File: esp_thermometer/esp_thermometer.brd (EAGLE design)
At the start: 50 x 50 mm, 11 parts, among them U2 DS18B20

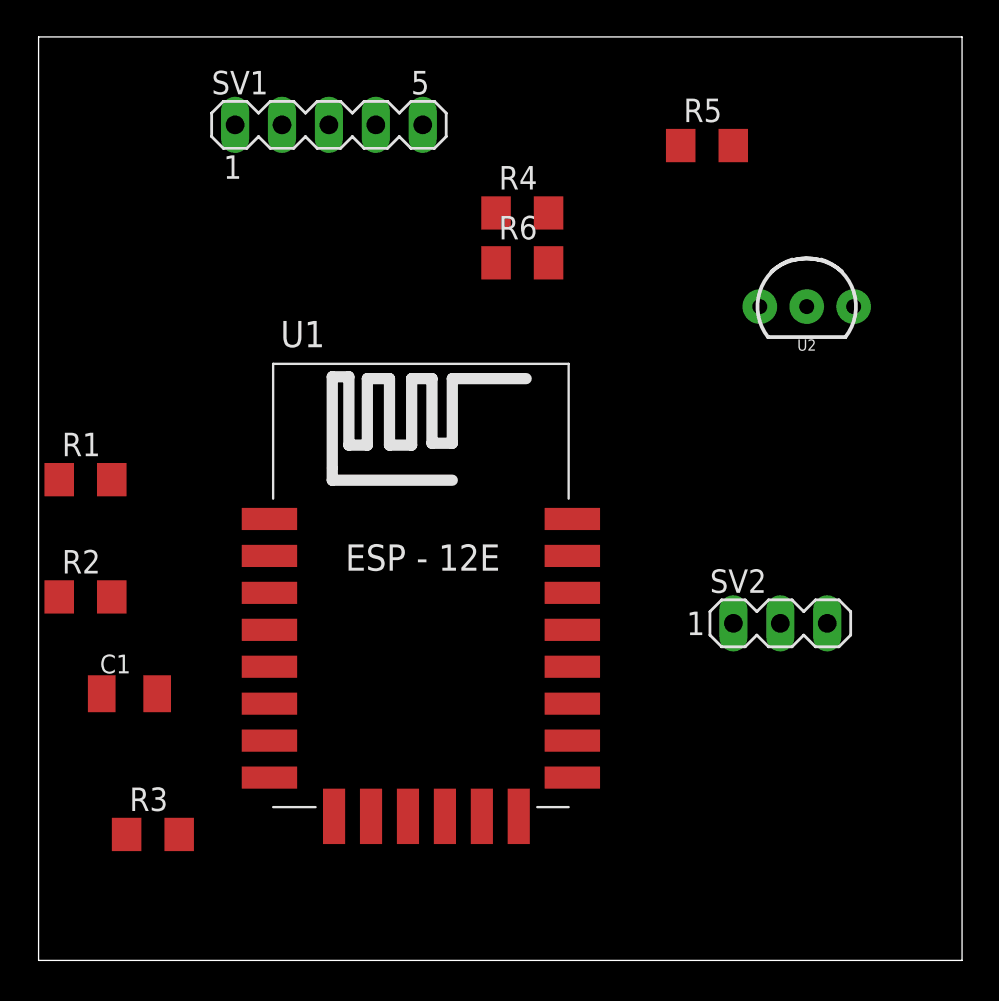
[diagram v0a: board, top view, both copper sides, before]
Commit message: Fertiger Schaltplan und Layout esp-thermometer
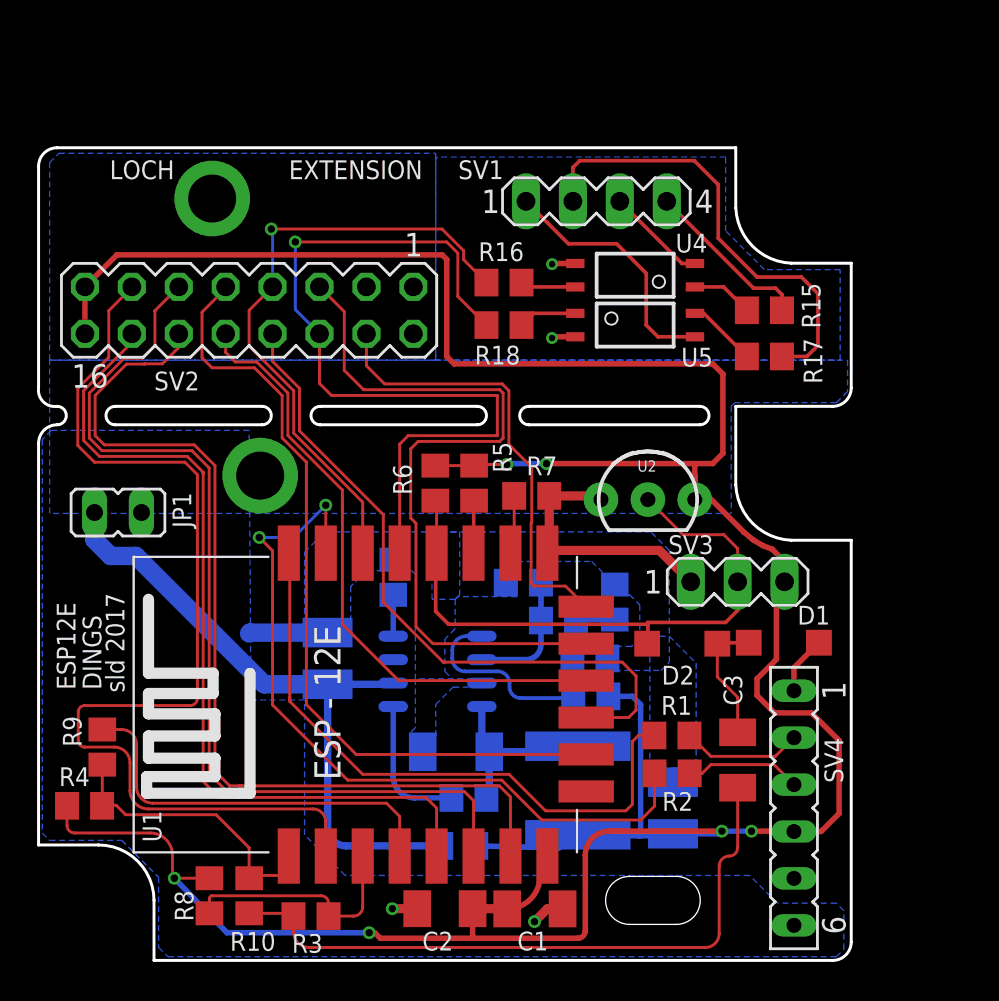
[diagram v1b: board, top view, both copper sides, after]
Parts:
- added C2: 1N00, rcl:C1206K
- added C3: 100n, rcl:C1206K
- added C4: 100N, rcl:C0805
- added C5: 47U0, rcl:C1210
- added C6: (no value), rcl:C1210
- added C7: 8N20, rcl:C0805
- added C8: 3N00, rcl:C0805
- added C9: 68N0, rcl:C0805
- added D1, D2: MBR0520LT, diode:SOD123
- added D3: SS24FL, slqlib:SOD-123_MINI-SMA
- added JP1: (no value), jumper:JP1
- added L1: SRN5020-220M, slqlib:L5050
- added R10, R13, R9: 0R00, rcl:R0805
- added R11, R15, R16, R17, R18: 10K2, rcl:R0805
- added R12: 3K24, rcl:R0805
- added R14: 10k2, rcl:R0805
- added R7, R8: 1K00, rcl:R0805
- added SV3: (no value), con-lstb:MA03-1
- added SV4: (no value), con-lsta:FE06
- added U3: TPS54231D, slqlib:D0008A
- added U4, U5: TLP183, slqlib:MINI-FLAT-4
- C1: value (none) -> 10N0
- R1, R2, R3: value (none) -> 0R00; device rcl:R1206 -> rcl:R0805
- R4, R5: value (none) -> 1K00; device rcl:R1206 -> rcl:R0805
- R6: value (none) -> 4K70; device rcl:R1206 -> rcl:R0805
- SV1: device con-lstb:MA05-1 -> con-lstb:MA04-1
- SV2: device con-lstb:MA03-1 -> con-lstb:MA08-2
- moved R4 39.9 mm to (2.49, 8.37)
- moved R1 34.6 mm to (34.3, 12.2)
- moved SV2 33.4 mm to (11.4, 35.2), turned to 180 degrees
- moved R2 33.2 mm to (34.3, 10.1)
- moved C1 24.9 mm to (26.9, 2.79)
- moved R5 22.2 mm to (23.6, 25.8), turned to 90 degrees
- moved SV1 15.1 mm to (30.2, 41.1)
- moved U2 13.5 mm to (33.0, 24.9)
- moved R6 12.8 mm to (21.5, 25.8), turned to 90 degrees
- moved R3 9.63 mm to (14.8, 2.40), turned to 180 degrees
- moved U1 4.40 mm to (19.4, 13.9), turned to 90 degrees
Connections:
- new net +3V3: C1.1, C2.1, C5.1, L1.2, R11.2, R13.2, R4.1, R5.2, R6.2, R8.1, SV2.15, SV2.16, SV3.3, SV4.4, U1.VCC, U2.3
- new net ADC: SV2.13, U1.ADC
- new net CH_PD: R3.1, R8.2, U1.CH_PD
- new net CS0: U1.CS0
- new net GPIO0: D2.A, R6.1, SV3.2, U1.GPIO0, U2.2
- new net GPIO10: SV2.10, U1.GPIO10
- new net GPIO12: SV2.11, U1.GPIO12
- new net GPIO13: SV2.12, U1.GPIO13
- new net GPIO14: SV2.14, U1.GPIO14
- new net GPIO4: R18.2, SV2.6, U1.GPIO4
- new net GPIO5: R16.2, SV2.7, U1.GPIO5
- new net GPIO9: SV2.8, U1.GPIO9
- new net MISO: SV2.9, U1.MISO
- new net MOSI: SV2.5, U1.MOSI
- new net N$1: R9.2, U1.GPIO16
- new net N$10: C3.1, R10.2, R3.2
- new net N$11: R15.1, SV1.4
- new net N$12: SV1.3, U4.2
- new net N$13: R11.1, R12.2, U3.5
- new net N$14: R17.1, SV1.2
- new net N$15: C7.1, U3.4
- new net N$16: C8.1, R14.1
- new net N$17: C9.1, R14.2, U3.6
- new net N$18: R17.2, U5.4
- new net N$19: R16.1, U4.4
- new net N$2: C4.1, U3.1
- new net N$20: SV1.1, U5.3
- new net N$21: R18.1, U5.1
- new net N$3: R5.1, U1.GPIO2
- new net N$4: R1.2, SV4.2
- new net N$5: R7.1, U1.GPIO15
- new net N$6: R15.2, U4.1
- new net N$7: R2.2, SV4.3
- new net N$8: D1.C, SV4.1
- new net N$9: C3.2, D1.A, D2.C
- new net PH: C4.2, D3.A, L1.1, U3.8
- new net RESET: R10.1, R4.2, R9.1, U1.RESET
- new net RX: R2.1, U1.RXD0
- new net SCLK: SV2.4, U1.SCLK
- new net TX: R1.1, U1.TXD0
- net GND: now also C1.2, C2.2, C5.2, C6.1, C7.2, C8.2, C9.2, D3.C, JP1.1, R12.1, R7.2, SV2.1, SV2.2, SV2.3, SV3.1, SV4.6, U1.GND, U3.7, U4.3, U5.2
- net VDD: now also C6.2, JP1.2, R13.1, U3.2; no longer U2.3
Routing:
- net +3V3: track 0.00 -> 175.5 mm, vias 0 -> 6
- net ADC: track 0.00 -> 55.3 mm
- net GPIO12: track 0.00 -> 52.6 mm
- net GPIO13: track 0.00 -> 52.2 mm
- net GPIO14: track 0.00 -> 47.3 mm
- net GPIO4: track 0.00 -> 45.2 mm, vias 0 -> 1
- net MISO: track 0.00 -> 43.1 mm
- net RX: track 0.00 -> 41.7 mm, vias 0 -> 2
- net MOSI: track 0.00 -> 41.2 mm
- net GPIO9: track 0.00 -> 37.1 mm
- net VDD: track 0.00 -> 35.3 mm
- net N$10: track 0.00 -> 35.3 mm
- net GPIO10: track 0.00 -> 34.3 mm
- net TX: track 0.00 -> 34.2 mm
- net GPIO5: track 0.00 -> 33.9 mm, vias 0 -> 1
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- added copper zone on layer 16, net GND
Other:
- board size 50 x 50 mm -> 44 x 44 mm
- board text added: "DINGS"
- board text added: "ESP12E"
- board text added: "EXTENSION"
- board text added: "LOCH"
- board text added: "sld 2017"
